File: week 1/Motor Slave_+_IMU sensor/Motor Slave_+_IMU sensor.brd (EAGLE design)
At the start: 100 x 100 mm, 8 parts

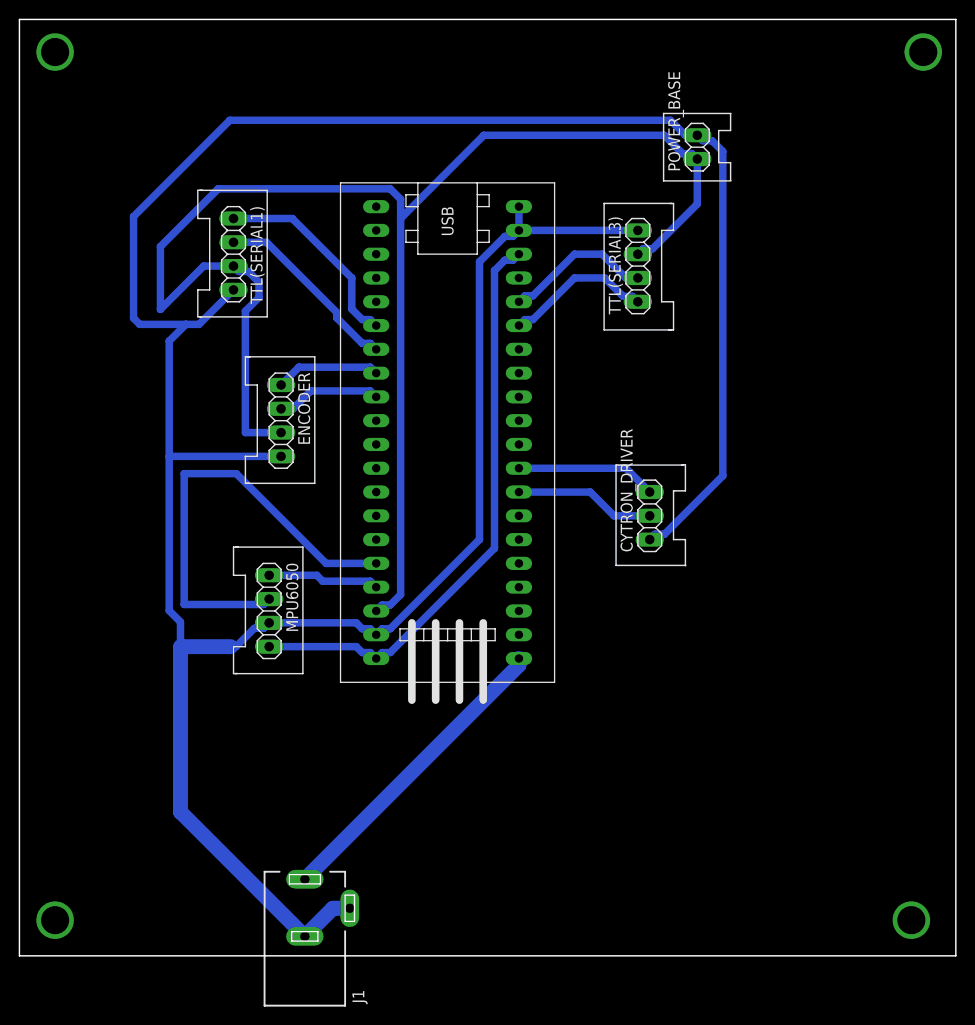
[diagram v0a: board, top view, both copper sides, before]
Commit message: .
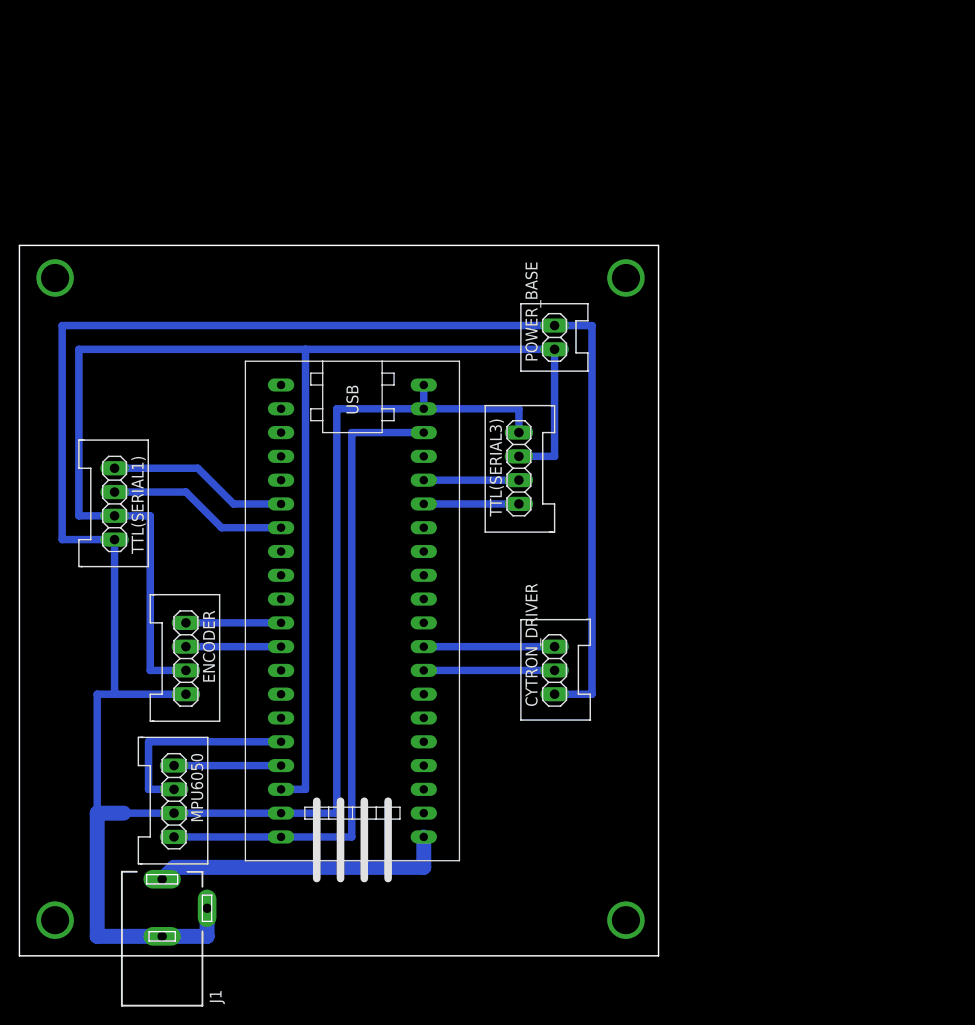
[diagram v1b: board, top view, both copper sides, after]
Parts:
- moved TTL(SERIAL1) 29.5 mm to (10.2, 48.3)
- moved ENCODER 27.4 mm to (17.8, 31.8)
- moved POWER_BASE 25.4 mm to (57.1, 66.0)
- moved TTL(SERIAL3) 25.0 mm to (53.3, 52.1)
- moved MPU6050 22.7 mm to (16.5, 16.5)
- moved U$1 21.6 mm to (35.6, 38.1)
- moved CYTRON_DRIVER 19.4 mm to (57.1, 30.5)
- moved J1 15.2 mm to (15.2, 5.08)
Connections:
- net PA_11: no longer ENCODER.1
- net PA_12: no longer ENCODER.2
- net PB_3: now also ENCODER.1
- net PB_4: now also ENCODER.2
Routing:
- net GND: track 315.5 -> 288.3 mm
- net PB_8: track 47.8 -> 22.0 mm
- net PA_12: track 11.2 -> 0.00 mm
- net PA_11: track 11.2 -> 0.00 mm
- net PB_4: track 0.00 -> 10.2 mm
- net PB_3: track 0.00 -> 10.2 mm
- net 3.3V: track 62.5 -> 69.9 mm
- net PB_11: track 15.9 -> 10.2 mm
- net PB_10: track 15.9 -> 10.2 mm
- net 5V: track 164.3 -> 161.4 mm
- net PA_9: track 21.9 -> 19.4 mm
- net VB: track 33.0 -> 31.7 mm
- net PA_3: track 15.0 -> 14.0 mm
- net PA_4: track 15.0 -> 14.0 mm
- net PA_10: track 20.3 -> 19.4 mm
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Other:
- board size 100 x 100 mm -> 68.2 x 75.9 mm
